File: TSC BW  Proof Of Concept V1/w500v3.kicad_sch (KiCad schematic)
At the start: 37 parts, among them J18 RJ45_Hanrun_HR911105A_Horizon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, U46 W5500, Y4 25M

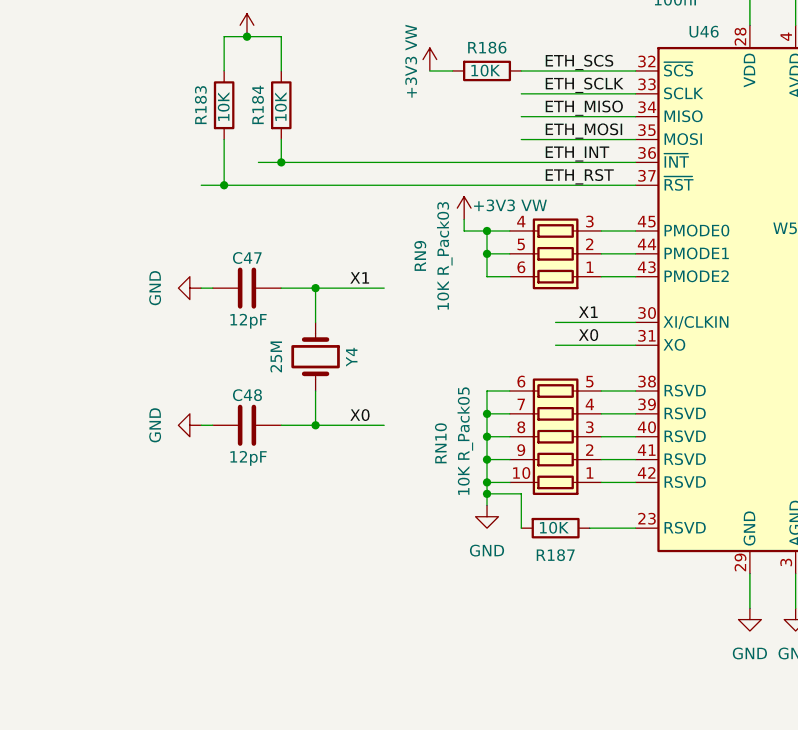
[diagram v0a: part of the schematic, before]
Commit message: WORKING ON POC - Proof of concept
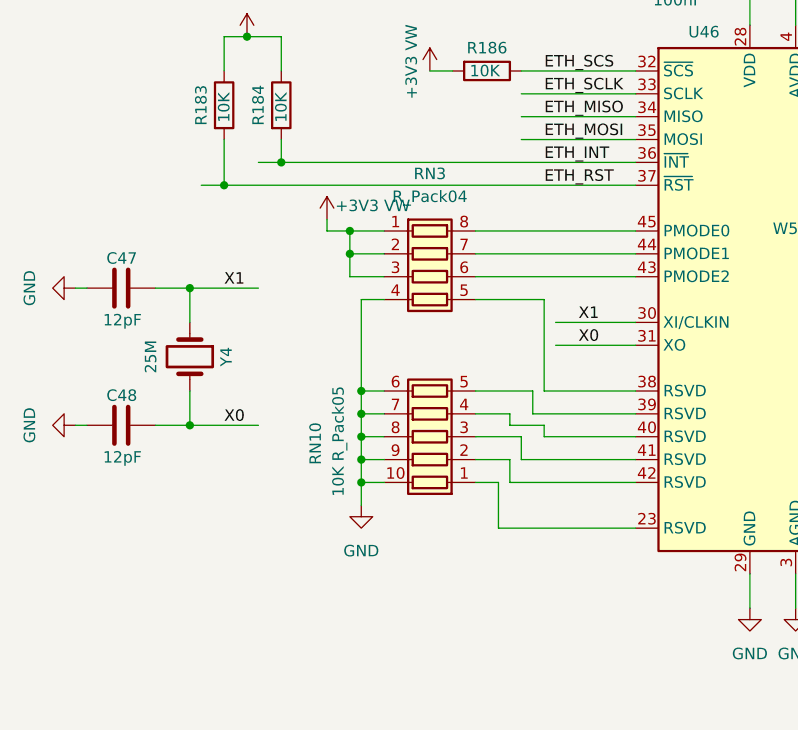
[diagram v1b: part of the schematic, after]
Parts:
- removed R187: 10K, Resistor_SMD:R_1206_3216Metric_Pad1.30x1.75mm_HandSolder, symbol Device:R
- removed RN9: 10K R_Pack03, symbol Device:R_Pack03
- added RN3: R_Pack04, Resistor_SMD:R_Array_Convex_4x1206, symbol Device:R_Pack04
- RN10: footprint (none) -> Resistor_SMD:R_Array_Convex_5x1206
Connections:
- net +3V3 VW: now also RN3.1 (R1.1), RN3.2 (R2.1), RN3.3 (R3.1)
- net GND: now also RN3.4 (R4.1)
- net at RN10.1 (R1.1): now also U46.23 (RSVD); no longer U46.42 (RSVD)
- net at RN10.2 (R2.1): now also U46.42 (RSVD); no longer U46.41 (RSVD)
- net at RN10.3 (R3.1): now also U46.41 (RSVD); no longer U46.40 (RSVD)
- net at RN10.4 (R4.1): now also U46.40 (RSVD); no longer U46.39 (RSVD)
- net at RN10.5 (R5.1): now also U46.39 (RSVD); no longer U46.38 (RSVD)
- net at U46.43 (PMODE2): now also RN3.6 (R3.2)
- net at U46.44 (PMODE1): now also RN3.7 (R2.2)
- net at U46.45 (PMODE0): now also RN3.8 (R1.2)
- new net: RN3.5 (R4.2), U46.38 (RSVD)
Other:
- moved on the sheet: C47, C48, RN10, Y4
